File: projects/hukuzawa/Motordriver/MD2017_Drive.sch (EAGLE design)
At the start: 3 parts

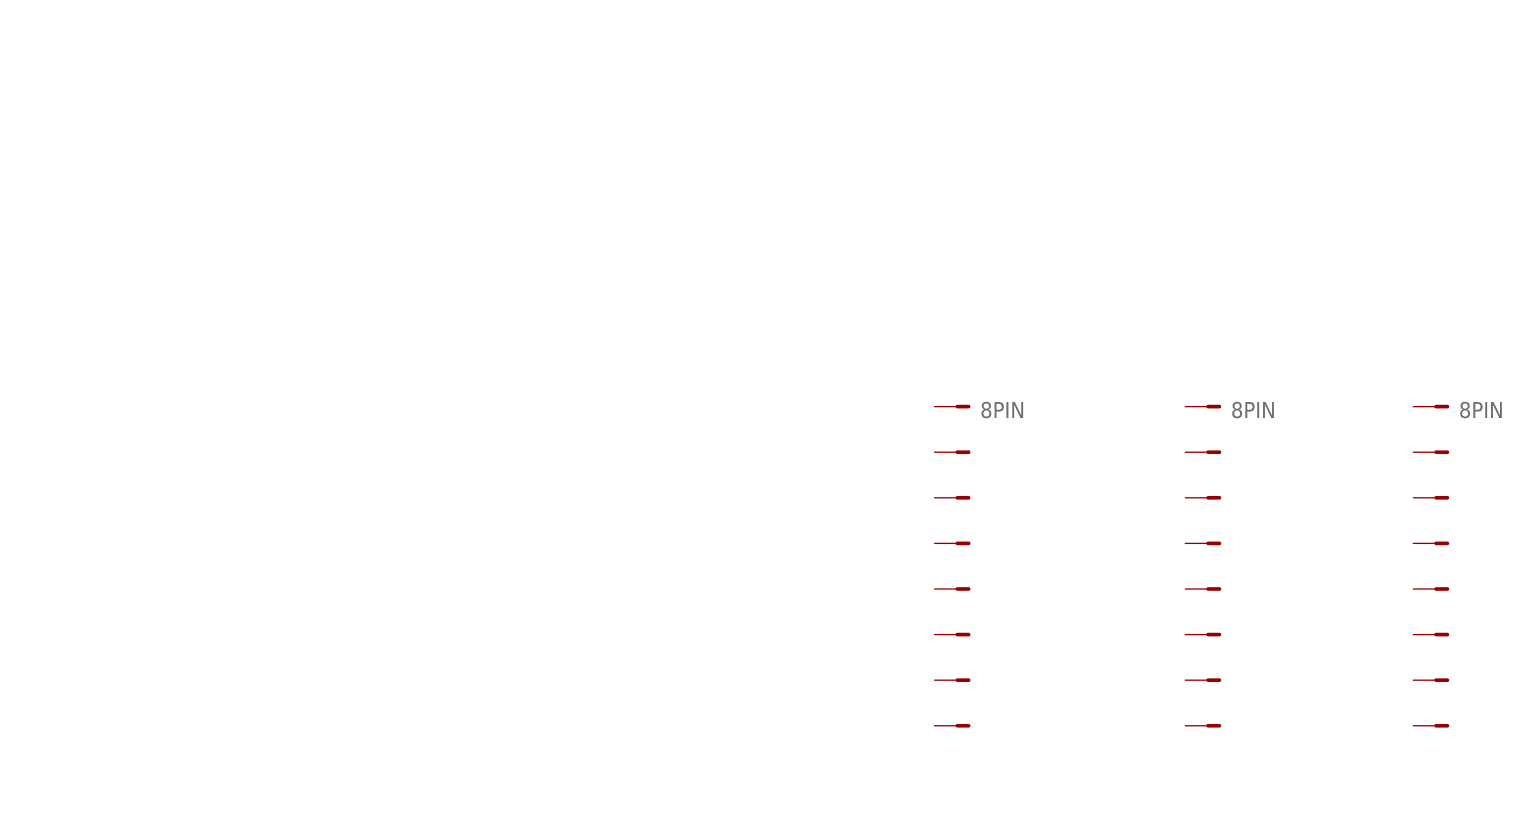
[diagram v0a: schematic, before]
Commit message: ドライバ駆動部回路図製作経過
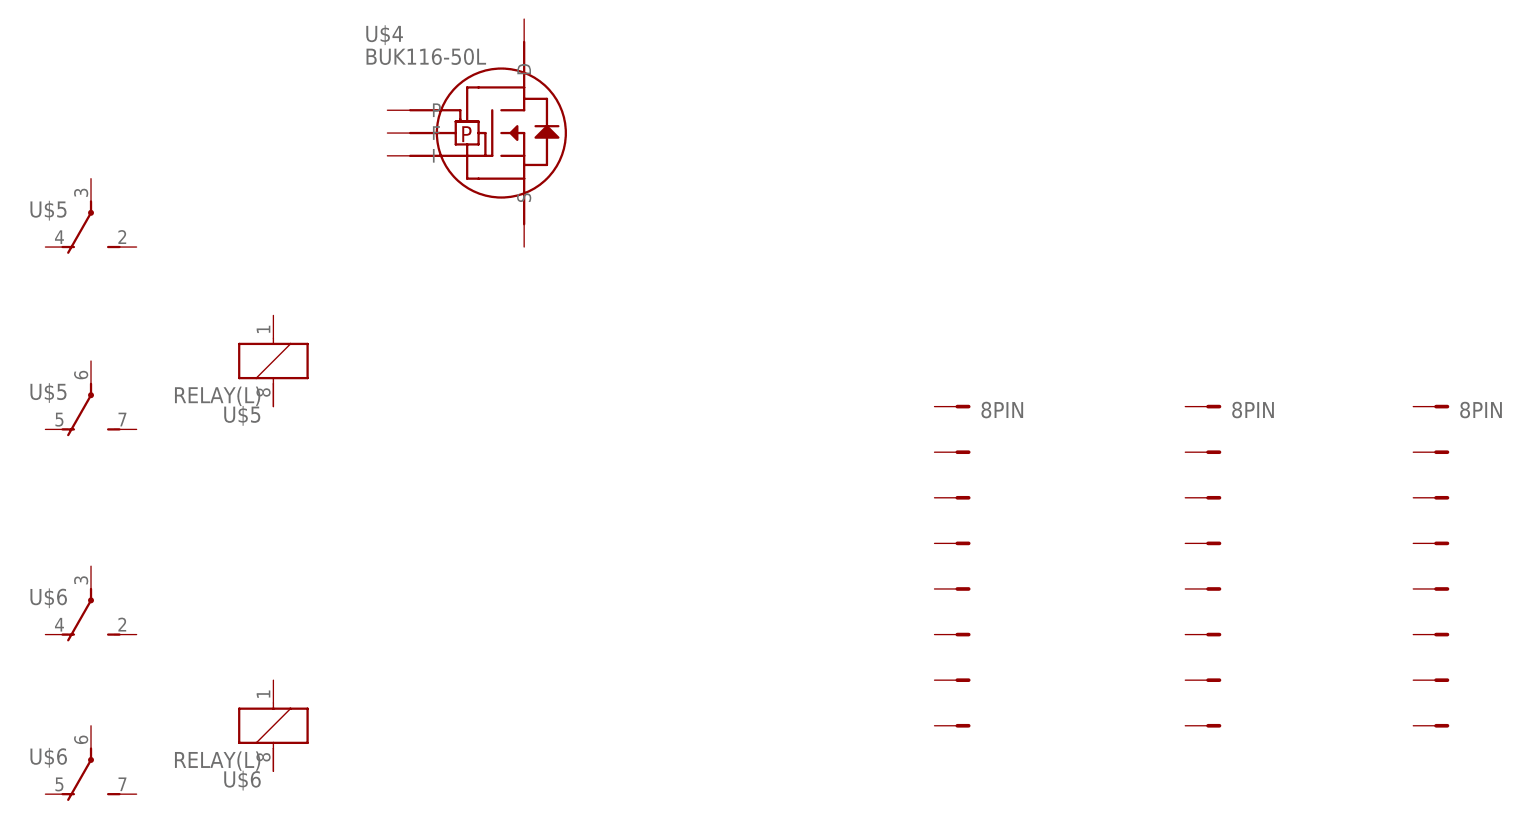
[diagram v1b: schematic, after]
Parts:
- added U$4: BUK116-50L, BUK116-50L:BUK116-50L
- added U$5, U$6: RELAY(L), relay:RELAY(L)
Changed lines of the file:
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@@
 <part name="U$2" library="FH105" deviceset="8PIN" device=""/>
 <part name="U$3" library="FH105" deviceset="8PIN" device=""/>
+<part name="U$4" library="BUK116-50L" deviceset="BUK116-50L" device=""/>
+<part name="U$5" library="relay" deviceset="RELAY(L)" device=""/>
+<part name="U$6" library="relay" deviceset="RELAY(L)" device=""/>
 </parts>
 <sheets>
@@
 <instance part="U$3" gate="-7" x="83.82" y="-25.4"/>
 <instance part="U$3" gate="-1" x="83.82" y="5.08"/>
+<instance part="U$4" gate="G$1" x="-22.86" y="35.56"/>
+<instance part="U$5" gate="R1" x="-68.58" y="5.08" rot="R180"/>
+<instance part="U$5" gate="1" x="-48.26" y="10.16" rot="R180"/>
+<instance part="U$5" gate="R2" x="-68.58" y="25.4" rot="R180"/>
+<instance part="U$6" gate="R1" x="-68.58" y="-35.56" rot="R180"/>
+<instance part="U$6" gate="1" x="-48.26" y="-30.48" rot="R180"/>
+<instance part="U$6" gate="R2" x="-68.58" y="-17.78" rot="R180"/>
 </instances>
 <busses>
